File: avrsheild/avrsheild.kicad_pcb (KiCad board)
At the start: 2 copper layers, 50 x 50 mm, 21 parts, among them J1 USB-C, J2 portD, J3 portC, J4 portB, SW1 SW_Push, U1 ATmega328P-P, U2 CH340C, Y1 Crystal

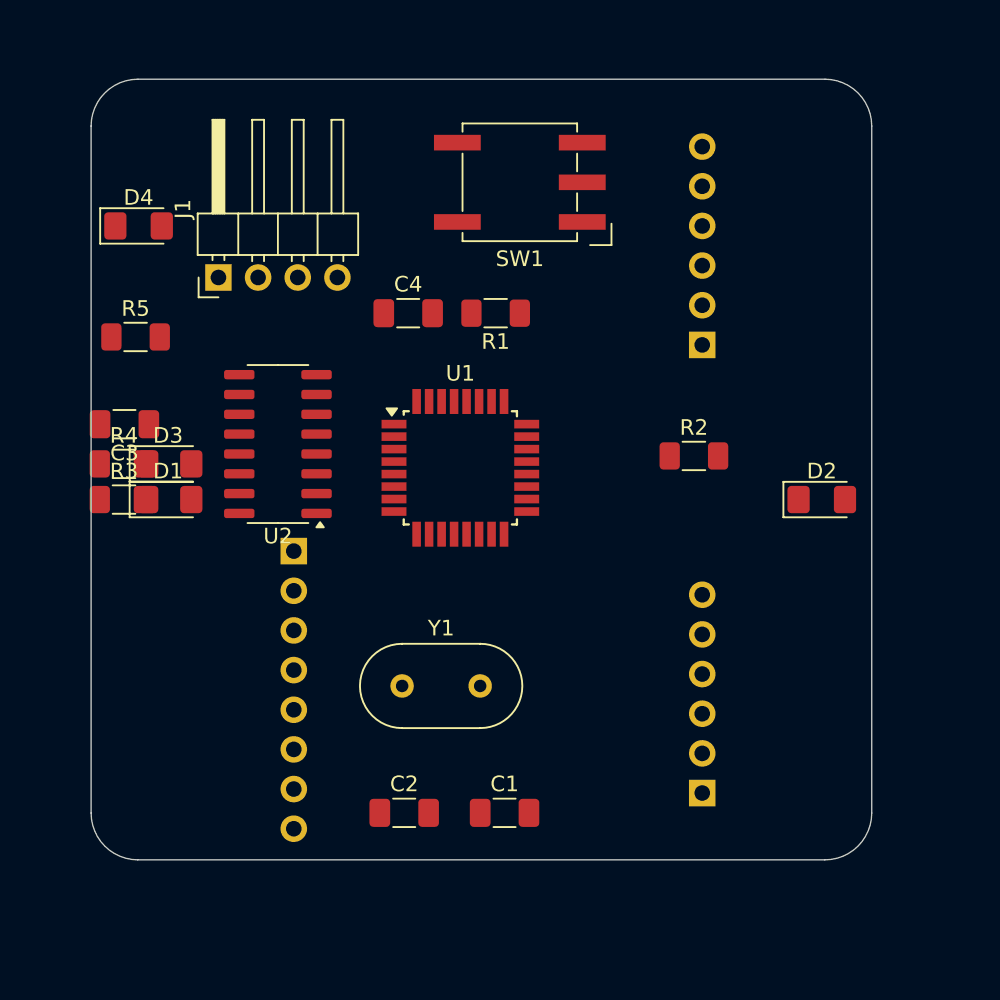
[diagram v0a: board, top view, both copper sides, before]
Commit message: PCB layout is done
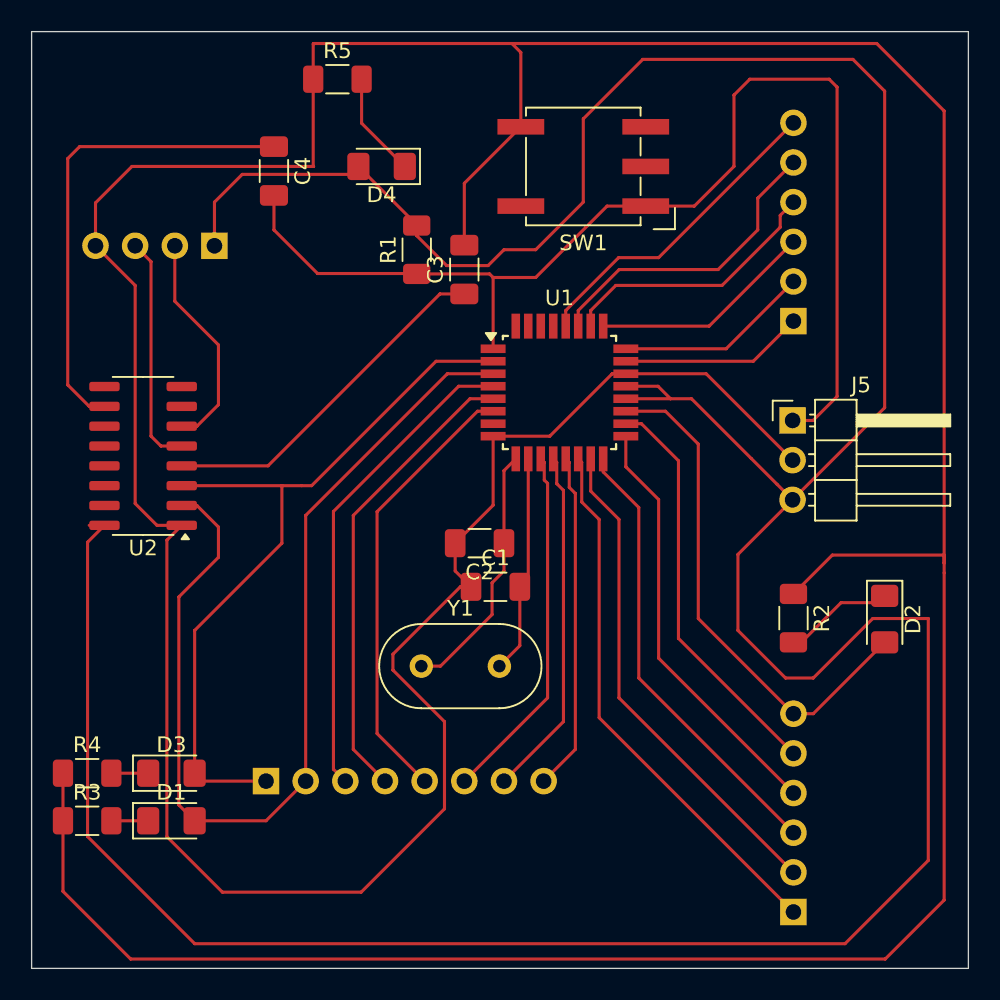
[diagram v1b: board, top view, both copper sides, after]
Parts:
- added J5: Power_pin, Connector_PinHeader_2.54mm:PinHeader_1x03_P2.54mm_Horizontal, F.Cu at (164.8, 62.2)
- J1: moved to B.Cu
- moved C3 23.9 mm to (143.8, 52.6), turned to 90 degrees
- moved R5 21.0 mm to (135.6, 40.4)
- moved R3 20.7 mm to (119.6, 87.9)
- moved D1 20.6 mm to (125.0, 87.9)
- moved R4 20.0 mm to (119.6, 84.8)
- moved D3 19.8 mm to (125.0, 84.8)
- moved C2 17.9 mm to (144.7, 70.1), turned to 180 degrees
- moved D4 16.0 mm to (138.5, 46.0), turned to 180 degrees
- moved J2 14.8 mm to (131.1, 85.3), turned to -90 degrees
- moved C1 14.5 mm to (145.8, 72.9)
- moved C4 12.5 mm to (131.6, 46.3), turned to -90 degrees
- moved R2 12.2 mm to (164.8, 74.9), turned to -90 degrees
- moved J4 9.60 mm to (164.8, 93.7)
- moved U2 8.67 mm to (123.2, 64.5)
- moved D2 8.65 mm to (170.7, 75.0), turned to -90 degrees
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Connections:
- C2 pad 1: Net-(D2-A) -> Net-(U1-XTAL1/PB6)
- U1 pad 9: Net-(D2-A) -> Net-(U1-XTAL1/PB6)
- U2 pad 5: Net-(J1-Pin_2) -> Net-(J1-Pin_3)
- U2 pad 6: Net-(J1-Pin_3) -> Net-(J1-Pin_2)
- Y1 pad 1: Net-(D2-A) -> Net-(U1-XTAL1/PB6)
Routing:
- net GND: track 0.00 -> 327.5 mm
- net +5V: track 0.00 -> 224.9 mm
- net Net-(J5-Pin_1): track 0.00 -> 75.6 mm
- net Net-(D1-A): track 0.00 -> 64.2 mm
- net Net-(D3-A): track 0.00 -> 48.8 mm
- net Net-(J4-Pin_1): track 0.00 -> 34.7 mm
- net Net-(D2-A): track 0.00 -> 33.0 mm
- net Net-(J4-Pin_2): track 0.00 -> 31.9 mm
- net Net-(J2-Pin_3): track 0.00 -> 31.1 mm
- net Net-(U2-~{DSR}): track 0.00 -> 30.9 mm
- net Net-(J2-Pin_4): track 0.00 -> 29.9 mm
- net Net-(J4-Pin_3): track 0.00 -> 29.0 mm
- net Net-(J2-Pin_5): track 0.00 -> 28.6 mm
- net Net-(J4-Pin_4): track 0.00 -> 27.3 mm
- net Net-(J4-Pin_5): track 0.00 -> 26.1 mm
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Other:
- board size 50 x 50 mm -> 60 x 60 mm
